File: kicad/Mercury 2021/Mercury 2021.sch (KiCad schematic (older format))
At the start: 0 parts

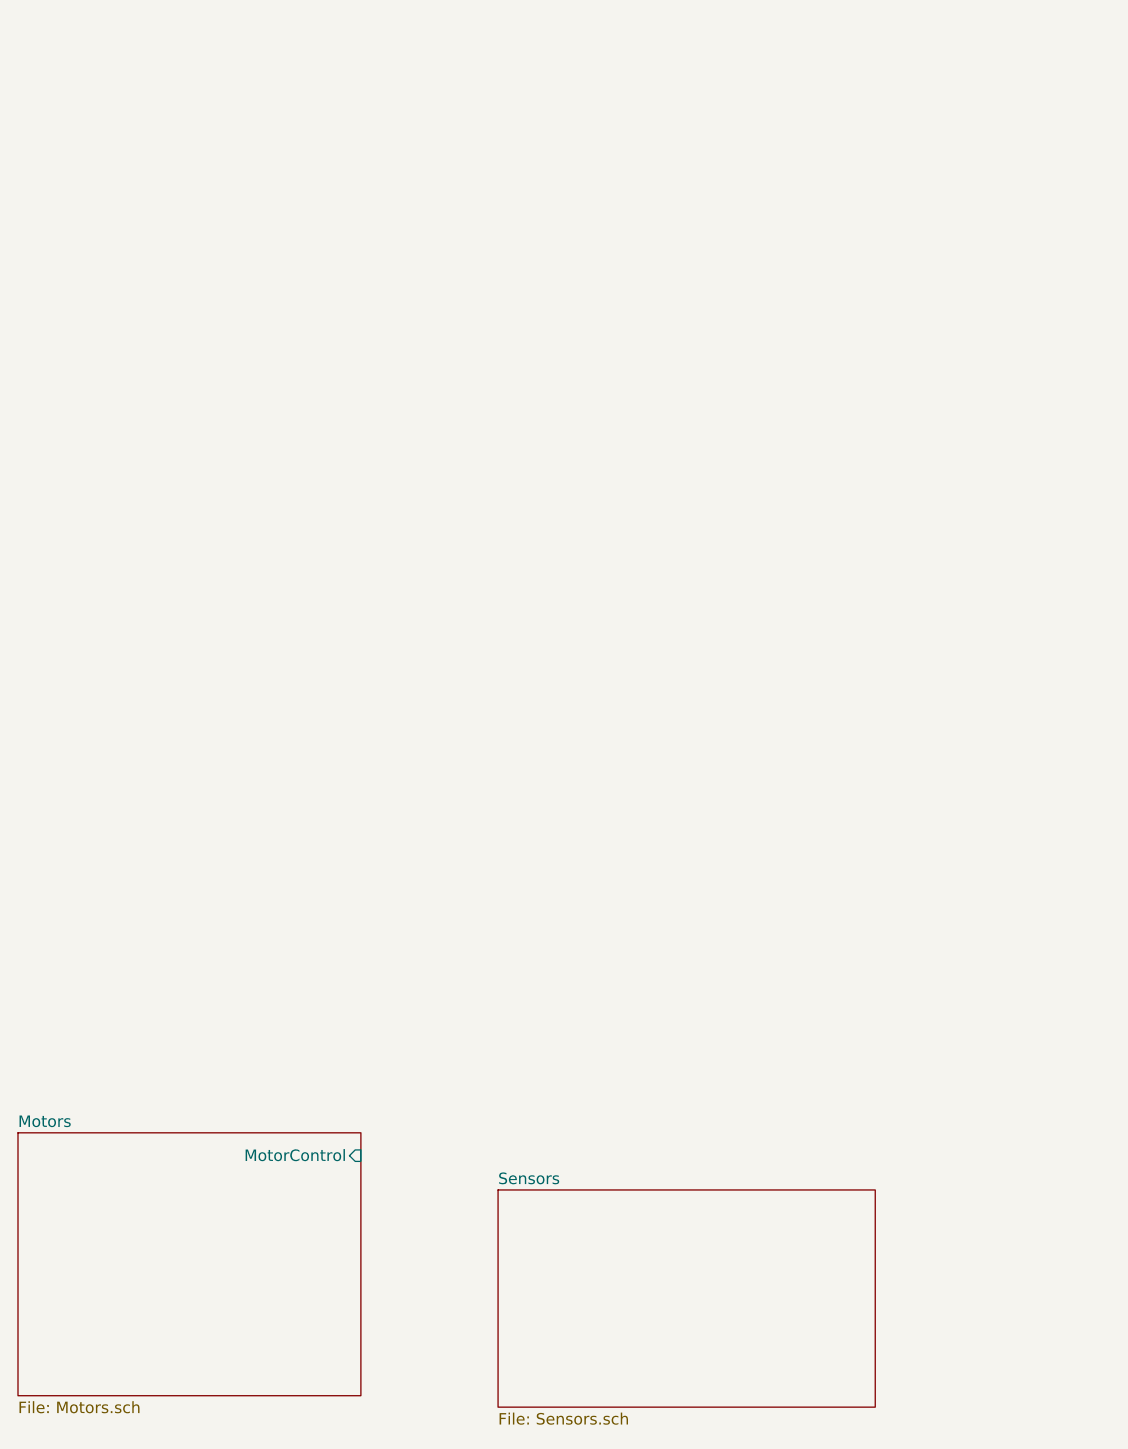
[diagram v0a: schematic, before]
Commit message: Updated new board
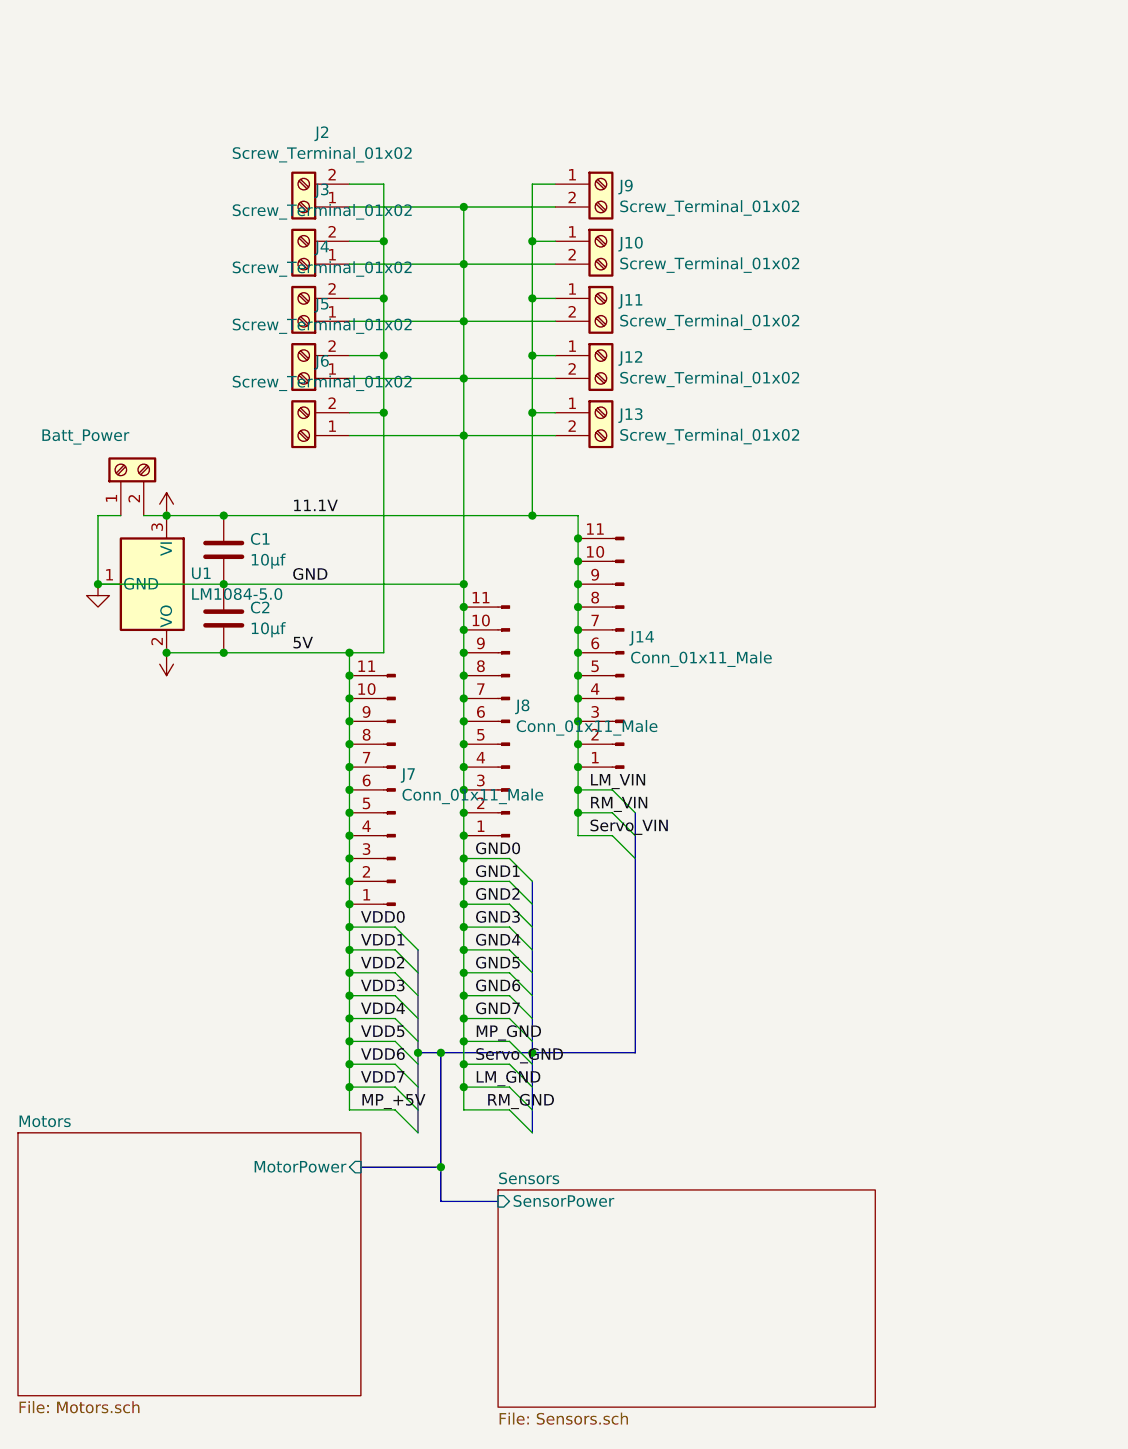
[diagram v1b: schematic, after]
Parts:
- added C1, C2: 10μf, symbol Device:C
- added J1: Batt_Power, symbol Connector:Screw_Terminal_01x02
- added J10, J11, J12, J13, J2, J3, J4, J5, J6, J9: Screw_Terminal_01x02, symbol Connector:Screw_Terminal_01x02
- added J14, J7, J8: Conn_01x11_Male, symbol Connector:Conn_01x11_Male
- added U1: LM1084-5.0, symbol Regulator_Linear:LM1084-5.0
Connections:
- new net +5V: C2.2, J2.2 (Pin_2), J3.2 (Pin_2), J4.2 (Pin_2), J5.2 (Pin_2), J6.2 (Pin_2), J7.1 (Pin_1), J7.10 (Pin_10), J7.11 (Pin_11), J7.2 (Pin_2), J7.3 (Pin_3), J7.4 (Pin_4), J7.5 (Pin_5), J7.6 (Pin_6), J7.7 (Pin_7), J7.8 (Pin_8), J7.9 (Pin_9), U1.2 (VO)
- new net +BATT: C1.1, J1.2 (Pin_2), J10.1 (Pin_1), J11.1 (Pin_1), J12.1 (Pin_1), J13.1 (Pin_1), J14.1 (Pin_1), J14.10 (Pin_10), J14.11 (Pin_11), J14.2 (Pin_2), J14.3 (Pin_3), J14.4 (Pin_4), J14.5 (Pin_5), J14.6 (Pin_6), J14.7 (Pin_7), J14.8 (Pin_8), J14.9 (Pin_9), J9.1 (Pin_1), U1.3 (VI)
- new net GND: C1.2, C2.1, J1.1 (Pin_1), J10.2 (Pin_2), J11.2 (Pin_2), J12.2 (Pin_2), J13.2 (Pin_2), J2.1 (Pin_1), J3.1 (Pin_1), J4.1 (Pin_1), J5.1 (Pin_1), J6.1 (Pin_1), J8.1 (Pin_1), J8.10 (Pin_10), J8.11 (Pin_11), J8.2 (Pin_2), J8.3 (Pin_3), J8.4 (Pin_4), J8.5 (Pin_5), J8.6 (Pin_6), J8.7 (Pin_7), J8.8 (Pin_8), J8.9 (Pin_9), J9.2 (Pin_2), U1.1 (GND)

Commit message: Updated new board
Created a 3.3v rail
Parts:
- removed C2: 10μf, symbol Device:C
- added C? (x3): 10μf, symbol Device:CP
- added J?: Conn_01x11_Male, symbol Connector:Conn_01x11_Male
- added J? (x5): Screw_Terminal_01x02, symbol Connector:Screw_Terminal_01x02
- added U?: LM1084-3.3, symbol Regulator_Linear:LM1084-3.3
- C1: symbol Device:C -> Device:CP
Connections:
- net +5V: now also J10.1 (Pin_1), J11.1 (Pin_1), J12.1 (Pin_1), J13.1 (Pin_1), J9.1 (Pin_1), C?.1; no longer J2.2 (Pin_2), J3.2 (Pin_2), J4.2 (Pin_2), J5.2 (Pin_2), J6.2 (Pin_2)
- net +BATT: now also C?.1, U?.3 (VI); no longer J10.1 (Pin_1), J11.1 (Pin_1), J12.1 (Pin_1), J13.1 (Pin_1), J9.1 (Pin_1)
- net GND: now also C?.2, J?.2 (Pin_2), J?.2 (Pin_2), J?.2 (Pin_2), J?.2 (Pin_2), J?.2 (Pin_2)
- new net: C?.2, C?.2
- new net +3V3: C?.1, J2.2 (Pin_2), J3.2 (Pin_2), J4.2 (Pin_2), J5.2 (Pin_2), J6.2 (Pin_2), J?.1 (Pin_1), J?.1 (Pin_1), J?.1 (Pin_1), J?.1 (Pin_1), J?.1 (Pin_1), J?.1 (Pin_1), J?.10 (Pin_10), J?.11 (Pin_11), J?.2 (Pin_2), J?.3 (Pin_3), J?.4 (Pin_4), J?.5 (Pin_5), J?.6 (Pin_6), J?.7 (Pin_7), J?.8 (Pin_8), J?.9 (Pin_9), U?.2 (VO)
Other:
- moved on the sheet: J10, J11, J12, J13, J2, J3, J4, J5, J6, J9
